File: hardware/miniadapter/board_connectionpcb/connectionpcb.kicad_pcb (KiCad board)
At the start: 2 copper layers, 10 x 6 mm, 11 parts

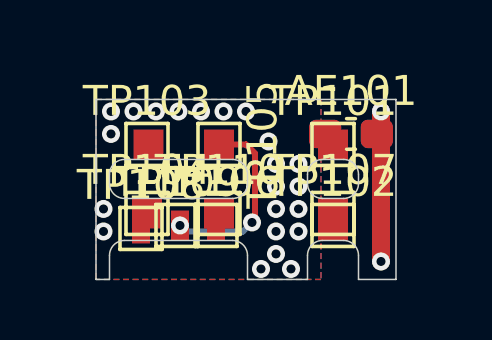
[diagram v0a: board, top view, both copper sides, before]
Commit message: new layout
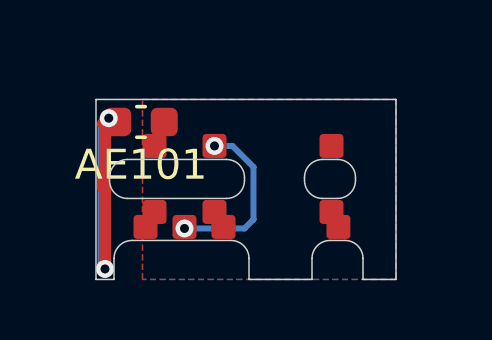
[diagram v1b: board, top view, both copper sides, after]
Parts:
- removed TP101, TP102, TP103, TP104, TP105, TP106, TP107, TP108, TP109, TP110: TestPoint, TestPoint:TestPoint_Pad_1.0x1.0mm
- added J101: Conn_01x04, minipcb:minipcb_alt_boardedge, B.Cu at (101.0, 101.5)
- added J102: Conn_02x03_Odd_Even, minipcb:ESP8685-WROOM-07, B.Cu at (100.5, 98.8)
- added REF**: Tab, PCM_kikit:Tab, F.Cu at (106.2, 96.1)
- added REF**: Tab, PCM_kikit:Tab, F.Cu at (110.0, 100.0)
- added REF**: Tab, PCM_kikit:Tab, F.Cu at (106.2, 102.1)
- added REF**: Tab, PCM_kikit:Tab, F.Cu at (100.0, 100.0)
- AE101: footprint Capacitor_SMD:C_0603_1608Metric_Pad1.08x0.95mm_HandSolder -> Capacitor_SMD:C_0603_1608Metric
- moved AE101 7.01 mm to (101.5, 96.8), turned to 180 degrees
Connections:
- AE101 pad 1: /ANT -> unconnected-(AE101-A-Pad1)
- AE101 pad 2: /GND -> unconnected-(AE101-Shield-Pad2)
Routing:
- net unconnected-(AE101-Shield-Pad2): track 0.00 -> 11.0 mm, vias 0 -> 2
- net /GND: track 10.8 -> 0.00 mm, vias 24 -> 0
- net Net-(TP105-Pad1): track 6.58 -> 0.00 mm, vias 2 -> 0
- net /IO5: track 0.00 -> 6.04 mm, vias 0 -> 2
- added copper zone on B.Cu, net unconnected-(AE101-Shield-Pad2)
- added copper zone on F.Cu, net unconnected-(AE101-Shield-Pad2)
- removed copper zone on B.Cu, net /GND
- removed copper zone on F.Cu, net /GND
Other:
- outline, holes or cut-outs redrawn
